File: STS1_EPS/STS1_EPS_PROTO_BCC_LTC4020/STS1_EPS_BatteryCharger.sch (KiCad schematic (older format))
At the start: 60 parts, among them J10 BG2, J11 BGATE, J3 Terminal BAT, J4 External NTC, J5 VIN_REG, J6 SHDN, J7 TG1, J8 TG2, J9 BG1, Q1 SI7135DP-T1-GE3, U1 LTC4020EUHF-PBF, U2 SI7272DP-T1-GE3, U3 SI7272DP-T1-GE3

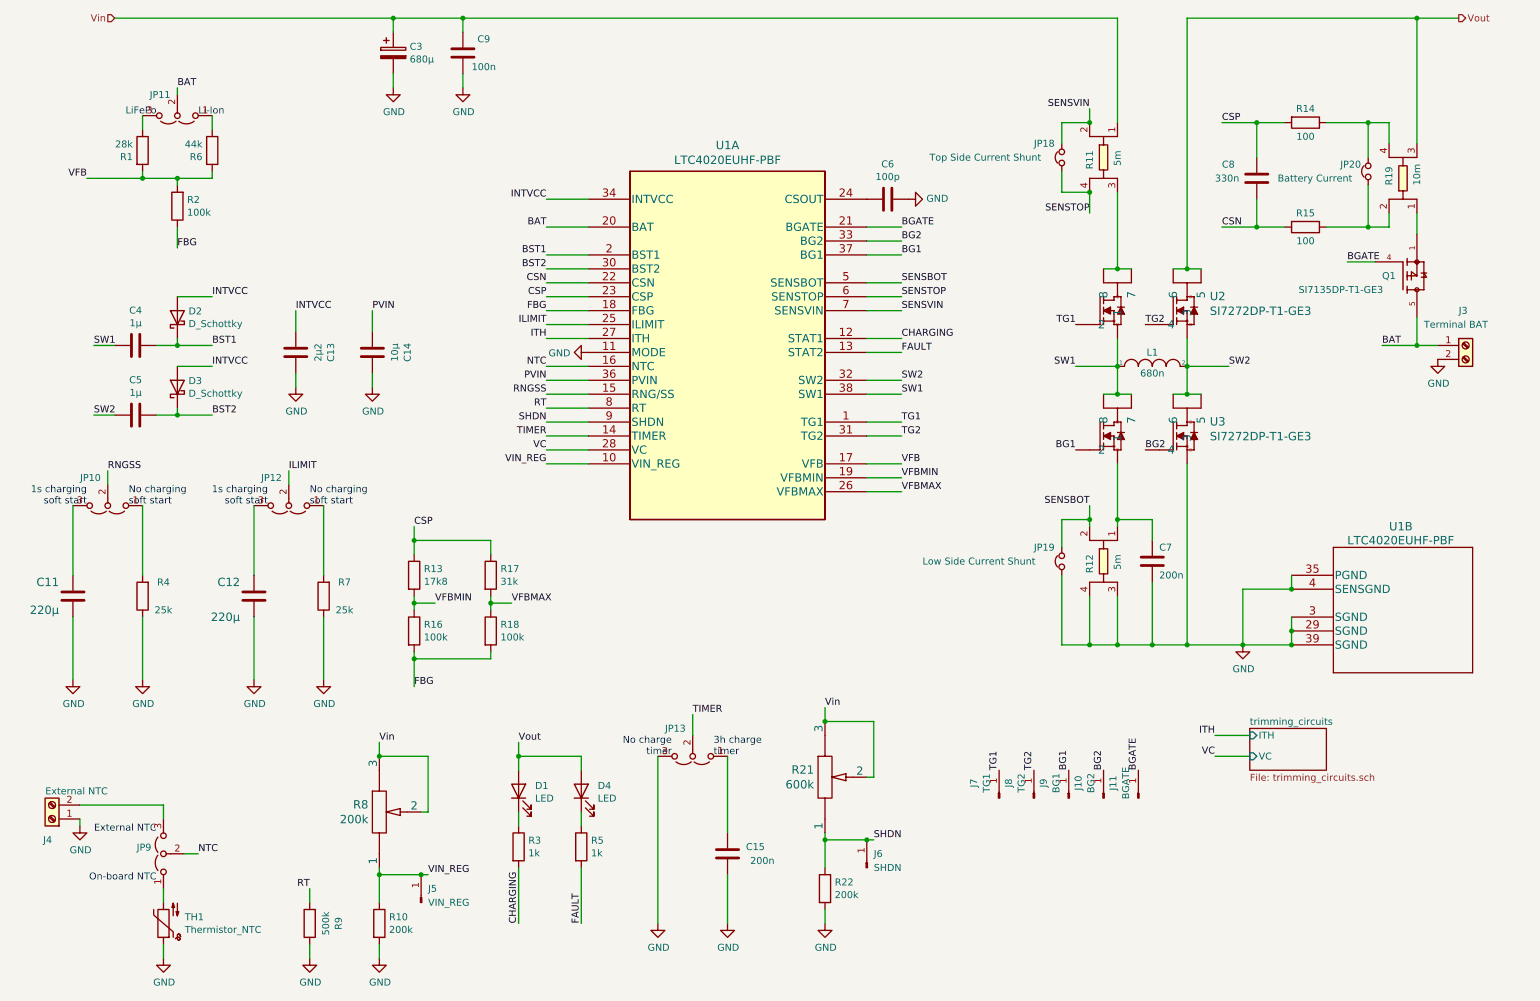
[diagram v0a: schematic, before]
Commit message: Intermediate state.
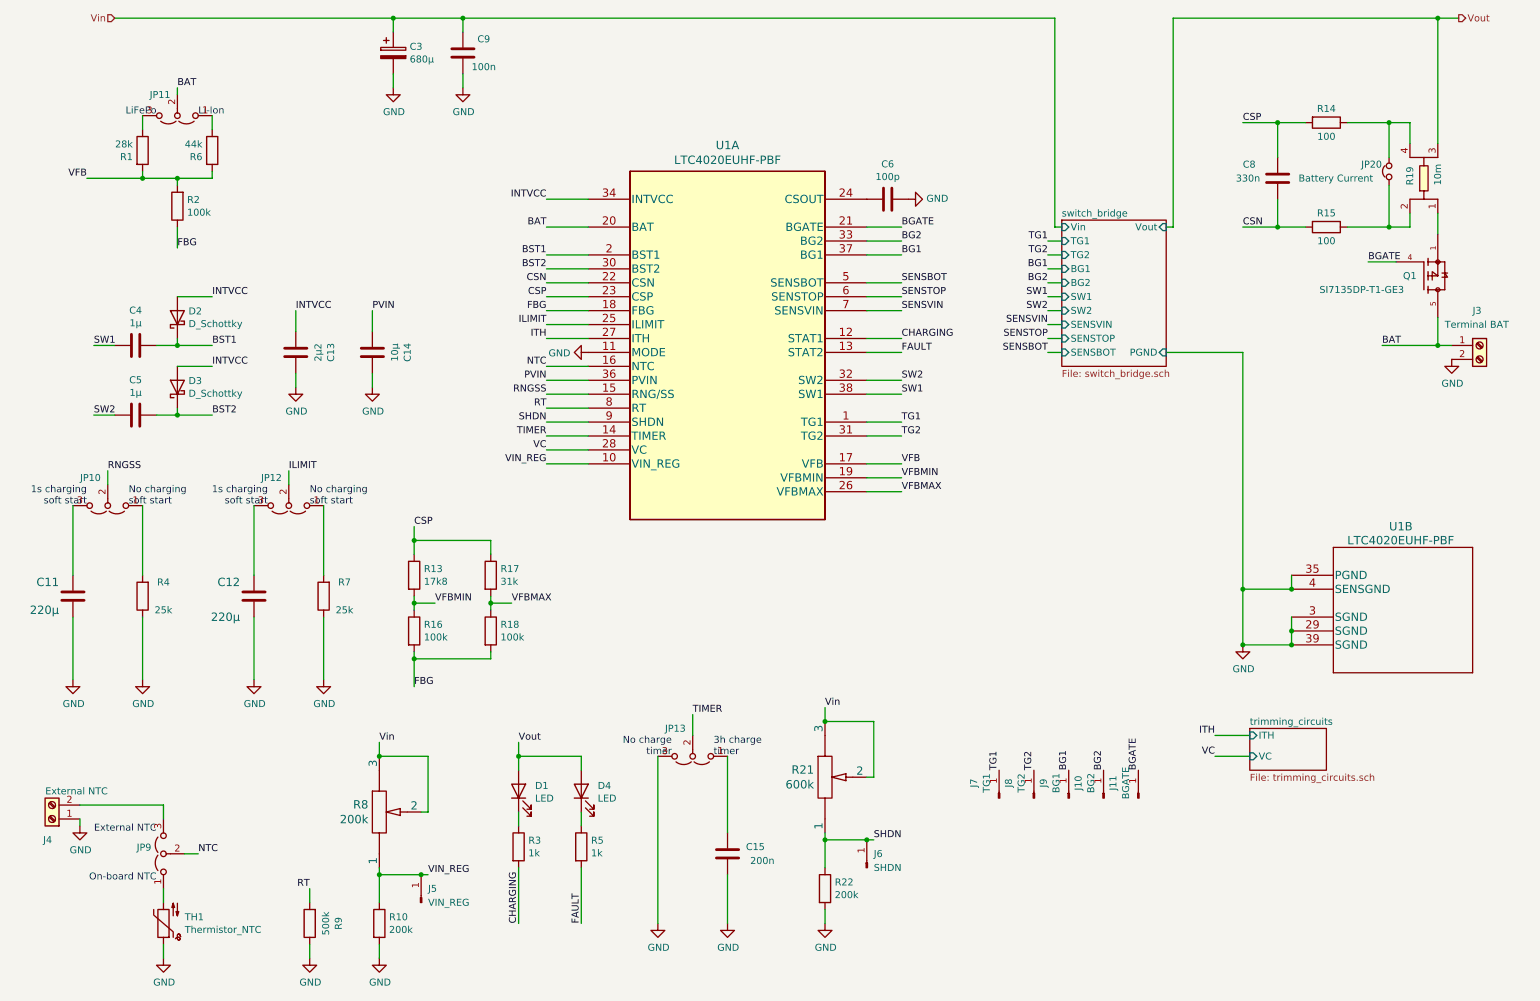
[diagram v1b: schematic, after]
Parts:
- removed C7: 200n, Capacitor_SMD:C_1812_4532Metric, symbol Device:C
- removed JP18: Top Side Current Shunt, Connector_PinHeader_2.54mm:PinHeader_1x02_P2.54mm_Vertical, symbol Device:Jumper_NC_Small
- removed JP19: Low Side Current Shunt, Connector_PinHeader_2.54mm:PinHeader_1x02_P2.54mm_Vertical, symbol Device:Jumper_NC_Small
- removed L1: 680n, footprints:INDPM7366X500N, symbol pspice:INDUCTOR
- removed R11, R12: 5m, footprints:CST0612-FC-R002E, symbol 2021-06-29_19-28-22:CST0612-FC-R002E
- removed U2, U3: SI7272DP-T1-GE3, footprints:SI7272DP-T1-GE3, symbol 2021-05-31_14-10-46:SI7272DP-T1-GE3
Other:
- moved on the sheet: C8, J3, JP20, Q1, R14, R15, R19
